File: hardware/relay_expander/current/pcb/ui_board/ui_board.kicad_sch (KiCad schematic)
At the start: 36 parts, among them J1 Conn_01x20_Socket

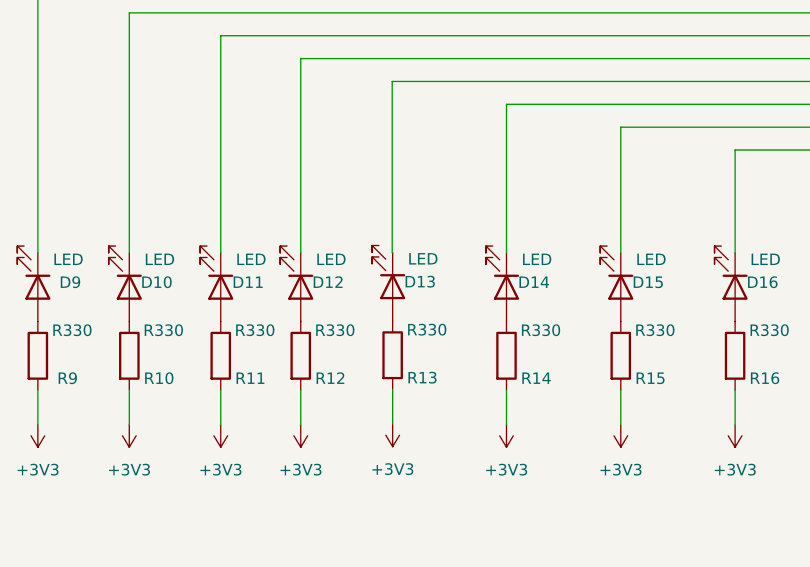
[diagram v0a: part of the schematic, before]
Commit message: [ADD] ui_board finished setup]
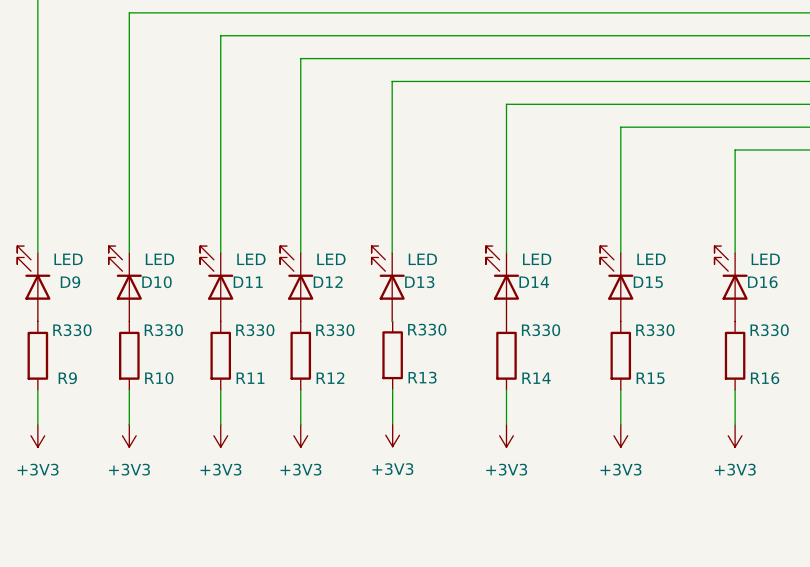
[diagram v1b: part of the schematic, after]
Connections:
- net at J1.17 (Pin_17): now also D13.1 (K)
